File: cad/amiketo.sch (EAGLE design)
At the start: 58 parts, among them CN1 MICROSDPLAIN, J1 HEADER-5X1, Q1 IRLML6344TRPBF, Q2 DMP2035U-7, SW2 SWITCHKMR211, SW3 SWITCHKMR211, U1 STM32F411/48, U2 LSM303D, U3 ADP5062, U4 MCP1824, U5 MAX17048, X1 12MHz, X2 32k768

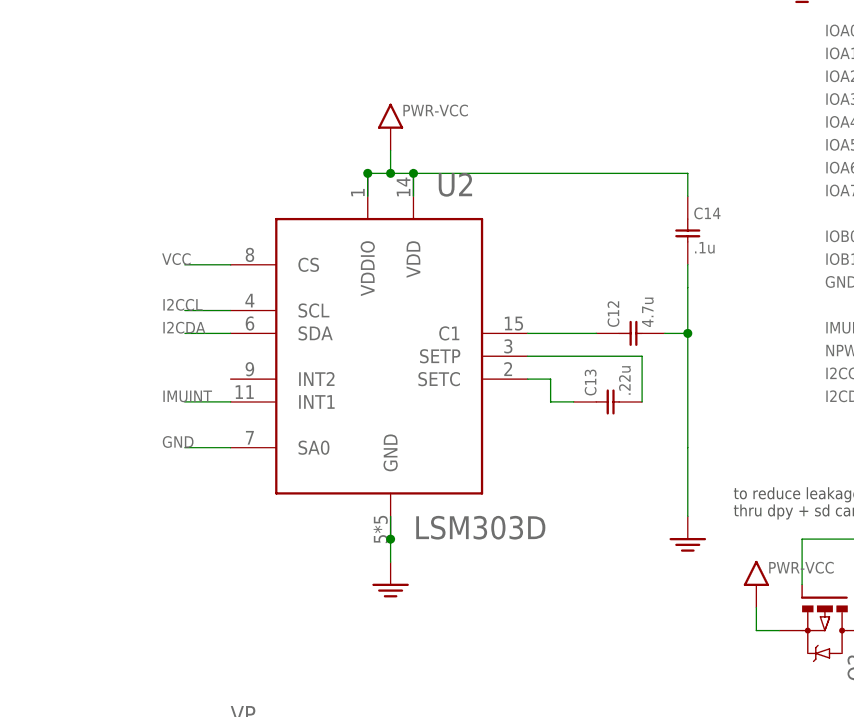
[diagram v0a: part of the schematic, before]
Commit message: lis3dh accel
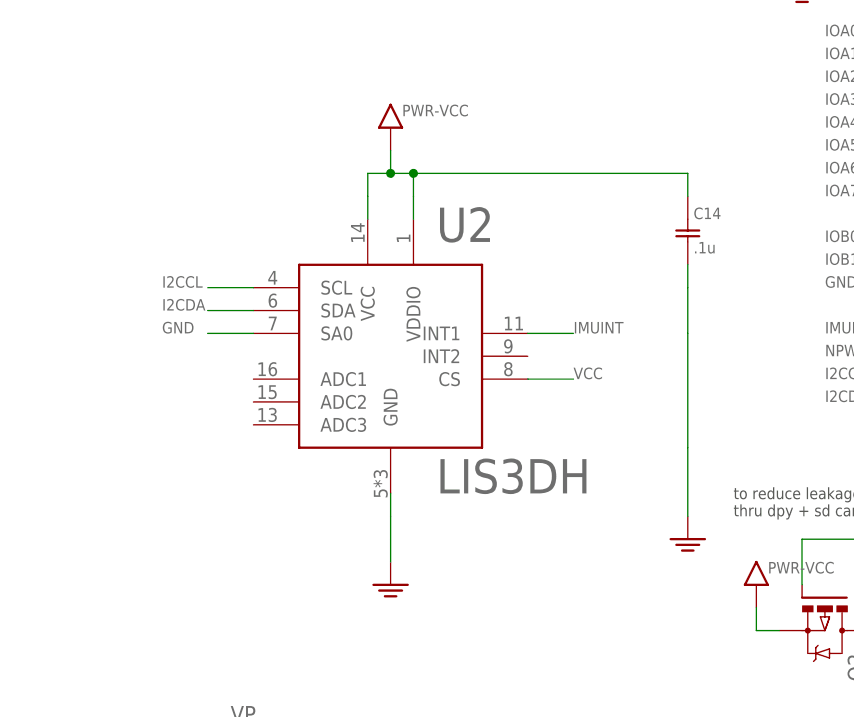
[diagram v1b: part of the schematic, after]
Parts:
- removed C12: 4.7u, jaw:C0603
- removed C13: .22u, jaw:C0603
- U2: value LSM303D -> LIS3DH; device jaw:LSM303D -> jaw:LIS3DH
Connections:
- removed net N$1: C12.P$1, U2.C1
- removed net N$2: C13.P$2, U2.SETP
- removed net N$4: C13.P$1, U2.SETC
- net GND: no longer C12.P$2
- net VCC: now also U2.VCC; no longer U2.VDD
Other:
- moved on the sheet: U2
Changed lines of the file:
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@@
 <part name="U$2" library="adafruit" deviceset="FIDUCIAL" device=""/>
 <part name="U$3" library="adafruit" deviceset="FIDUCIAL" device=""/>
-<part name="C12" library="jaw" deviceset="C" device="0603" value="4.7u"/>
-<part name="C13" library="jaw" deviceset="C" device="0603" value=".22u"/>
 <part name="C14" library="jaw" deviceset="C" device="0603" value=".1u"/>
 <part name="GND12" library="jaw" deviceset="PWR-GND" device=""/>
@@
 <part name="B1" library="jaw" deviceset="BATTERY" device="-CR2016"/>
 <part name="X1" library="jaw" deviceset="RESONATOR" device="CTCE" value="12MHz"/>
-<part name="U2" library="jaw" deviceset="LSM303D" device=""/>
 <part name="U5" library="jaw" deviceset="MAX17048" device=""/>
 <part name="LOGO1" library="Sparkfun-Aesthetics" deviceset="OSHW-LOGO" device="M"/>
@@
 <part name="C6" library="jaw" deviceset="C" device="0603" value="1u"/>
 <part name="C7" library="jaw" deviceset="C" device="0603" value="1u"/>
+<part name="U2" library="jaw" deviceset="LIS3DH" device=""/>
 </parts>
 <sheets>
@@
 <instance part="U$2" gate="G$1" x="269.24" y="40.64"/>
 <instance part="U$3" gate="G$1" x="261.62" y="40.64"/>
-<instance part="C12" gate="G$1" x="127" y="109.22" rot="R90"/>
-<instance part="C13" gate="G$1" x="124.46" y="101.6" rot="R90"/>
 <instance part="C14" gate="G$1" x="132.08" y="119.38"/>
 <instance part="GND12" gate="G$1" x="99.06" y="81.28"/>
@@
 <instance part="B1" gate="G$1" x="226.06" y="170.18"/>
 <instance part="X1" gate="G$1" x="144.78" y="160.02"/>
-<instance part="U2" gate="G$1" x="99.06" y="106.68"/>
 <instance part="U5" gate="G$1" x="127" y="25.4"/>
 <instance part="LOGO1" gate="G$1" x="203.2" y="45.72"/>
@@
 <instance part="C6" gate="G$1" x="226.06" y="73.66"/>
 <instance part="C7" gate="G$1" x="226.06" y="165.1" rot="R270"/>
+<instance part="U2" gate="G$1" x="99.06" y="106.68"/>
 </instances>
 <busses>
@@
 <pinref part="GND12" gate="G$1" pin="GND"/>
 <wire x1="99.06" y1="88.9" x2="99.06" y2="86.36" width="0.1524" layer="91"/>
+<wire x1="99.06" y1="86.36" x2="99.06" y2="83.82" width="0.1524" layer="91"/>
 <pinref part="U2" gate="G$1" pin="GND"/>
-<wire x1="99.06" y1="86.36" x2="99.06" y2="83.82" width="0.1524" layer="91"/>
-<junction x="99.06" y="86.36"/>
-</segment>
-<segment>
-<pinref part="C12" gate="G$1" pin="P$2"/>
-<wire x1="129.54" y1="109.22" x2="132.08" y2="109.22" width="0.1524" layer="91"/>
+<wire x1="99.06" y1="88.9" x2="99.06" y2="91.44" width="0.1524" layer="91"/>
+</segment>
+<segment>
 <wire x1="132.08" y1="109.22" x2="132.08" y2="96.52" width="0.1524" layer="91"/>
 <pinref part="GND14" gate="G$1" pin="GND"/>
 <wire x1="132.08" y1="96.52" x2="132.08" y2="88.9" width="0.1524" layer="91"/>
 <wire x1="132.08" y1="114.3" x2="132.08" y2="109.22" width="0.1524" layer="91"/>
-<junction x="132.08" y="109.22"/>
 <pinref part="C14" gate="G$1" pin="P$2"/>
 <wire x1="132.08" y1="116.84" x2="132.08" y2="114.3" width="0.1524" layer="91"/>
@@
 </segment>
 <segment>
-<pinref part="U2" gate="G$1" pin="SA0"/>
-<wire x1="81.28" y1="96.52" x2="76.2" y2="96.52" width="0.1524" layer="91"/>
-<label x="73.66" y="96.52" size="1.27" layer="95"/>
-</segment>
-<segment>
 <pinref part="U5" gate="G$1" pin="QSTRT"/>
 <wire x1="142.24" y1="22.86" x2="147.32" y2="22.86" width="0.1524" layer="91"/>
@@
 <pinref part="GND24" gate="G$1" pin="GND"/>
 <wire x1="264.16" y1="68.58" x2="256.54" y2="68.58" width="0.1524" layer="91"/>
+</segment>
+<segment>
+<pinref part="U2" gate="G$1" pin="SA0"/>
+<wire x1="83.82" y1="109.22" x2="78.74" y2="109.22" width="0.1524" layer="91"/>
+<label x="73.66" y="109.22" size="1.27" layer="95"/>
 </segment>
 </net>
@@
 <junction x="99.06" y="127"/>
 <pinref part="U2" gate="G$1" pin="VDDIO"/>
-<junction x="96.52" y="127"/>
-<pinref part="U2" gate="G$1" pin="VDD"/>
+<wire x1="101.6" y1="124.46" x2="101.6" y2="121.92" width="0.1524" layer="91"/>
+<pinref part="U2" gate="G$1" pin="VCC"/>
+<wire x1="96.52" y1="124.46" x2="96.52" y2="121.92" width="0.1524" layer="91"/>
 </segment>
 <segment>
@@
 <label x="246.38" y="177.8" size="1.27" layer="95"/>
 <pinref part="J1" gate="G$1" pin="1"/>
-</segment>
-<segment>
-<pinref part="U2" gate="G$1" pin="CS"/>
-<wire x1="81.28" y1="116.84" x2="76.2" y2="116.84" width="0.1524" layer="91"/>
-<label x="73.66" y="116.84" size="1.27" layer="95"/>
 </segment>
 <segment>
@@
 <wire x1="139.7" y1="78.74" x2="139.7" y2="76.2" width="0.1524" layer="91"/>
 <wire x1="139.7" y1="76.2" x2="142.24" y2="76.2" width="0.1524" layer="91"/>
+</segment>
+<segment>
+<pinref part="U2" gate="G$1" pin="CS"/>
+<wire x1="114.3" y1="104.14" x2="119.38" y2="104.14" width="0.1524" layer="91"/>
+<label x="119.38" y="104.14" size="1.27" layer="95"/>
 </segment>
 </net>
@@
 </segment>
 <segment>
-<pinref part="U2" gate="G$1" pin="SCL"/>
-<wire x1="81.28" y1="111.76" x2="76.2" y2="111.76" width="0.1524" layer="91"/>
-<label x="73.66" y="111.76" size="1.27" layer="95"/>
-</segment>
-<segment>
 <pinref part="U5" gate="G$1" pin="SCL"/>
 <wire x1="142.24" y1="27.94" x2="147.32" y2="27.94" width="0.1524" layer="91"/>
@@
 <label x="243.84" y="101.6" size="1.27" layer="95"/>
 </segment>
+<segment>
+<pinref part="U2" gate="G$1" pin="SCL"/>
+<wire x1="83.82" y1="114.3" x2="78.74" y2="114.3" width="0.1524" layer="91"/>
+<label x="73.66" y="114.3" size="1.27" layer="95"/>
+</segment>
 </net>
 <net name="I2CDA" class="0">
@@
 </segment>
 <segment>
-<pinref part="U2" gate="G$1" pin="SDA"/>
-<wire x1="81.28" y1="109.22" x2="76.2" y2="109.22" width="0.1524" layer="91"/>
-<label x="73.66" y="109.22" size="1.27" layer="95"/>
-</segment>
-<segment>
 <pinref part="U5" gate="G$1" pin="SDA"/>
 <wire x1="142.24" y1="30.48" x2="147.32" y2="30.48" width="0.1524" layer="91"/>
@@
 <label x="243.84" y="99.06" size="1.27" layer="95"/>
 </segment>
+<segment>
+<pinref part="U2" gate="G$1" pin="SDA"/>
+<wire x1="83.82" y1="111.76" x2="78.74" y2="111.76" width="0.1524" layer="91"/>
+<label x="73.66" y="111.76" size="1.27" layer="95"/>
+</segment>
 </net>
 <net name="DPYDC" class="0">
@@
 <segment>
 <pinref part="U2" gate="G$1" pin="INT1"/>
-<wire x1="81.28" y1="101.6" x2="76.2" y2="101.6" width="0.1524" layer="91"/>
-<label x="73.66" y="101.6" size="1.27" layer="95"/>
+<wire x1="114.3" y1="109.22" x2="119.38" y2="109.22" width="0.1524" layer="91"/>
+<label x="119.38" y="109.22" size="1.27" layer="95"/>
 </segment>
 </net>
@@
 </segment>
 </net>
-<net name="N$1" class="0">
-<segment>
-<pinref part="C12" gate="G$1" pin="P$1"/>
-<pinref part="U2" gate="G$1" pin="C1"/>
-<wire x1="121.92" y1="109.22" x2="114.3" y2="109.22" width="0.1524" layer="91"/>
-</segment>
-</net>
-<net name="N$2" class="0">
-<segment>
-<pinref part="U2" gate="G$1" pin="SETP"/>
-<wire x1="114.3" y1="106.68" x2="127" y2="106.68" width="0.1524" layer="91"/>
-<pinref part="C13" gate="G$1" pin="P$2"/>
-<wire x1="127" y1="106.68" x2="127" y2="101.6" width="0.1524" layer="91"/>
-</segment>
-</net>
-<net name="N$4" class="0">
-<segment>
-<pinref part="C13" gate="G$1" pin="P$1"/>
-<wire x1="119.38" y1="101.6" x2="116.84" y2="101.6" width="0.1524" layer="91"/>
-<wire x1="116.84" y1="101.6" x2="116.84" y2="104.14" width="0.1524" layer="91"/>
-<pinref part="U2" gate="G$1" pin="SETC"/>
-<wire x1="116.84" y1="104.14" x2="114.3" y2="104.14" width="0.1524" layer="91"/>
-</segment>
-</net>
